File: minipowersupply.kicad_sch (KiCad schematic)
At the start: 43 parts, among them J1 Conn_01x08_Female, J2 Conn_01x08_Female, J3 Conn_01x03_Female, J4 Conn_01x08_Female, J5 Conn_01x03_Female, J6 Conn_01x08_Female, J7 Conn_01x03_Female, J8 Conn_01x02_Female, J9 Conn_01x02_Female, Q1 BC817, U1 LM7805_TO220, U15 LT1084-3.3, U2 LM317L_TO92, U3 LM337L_TO92, U4 CD74HC4067SM

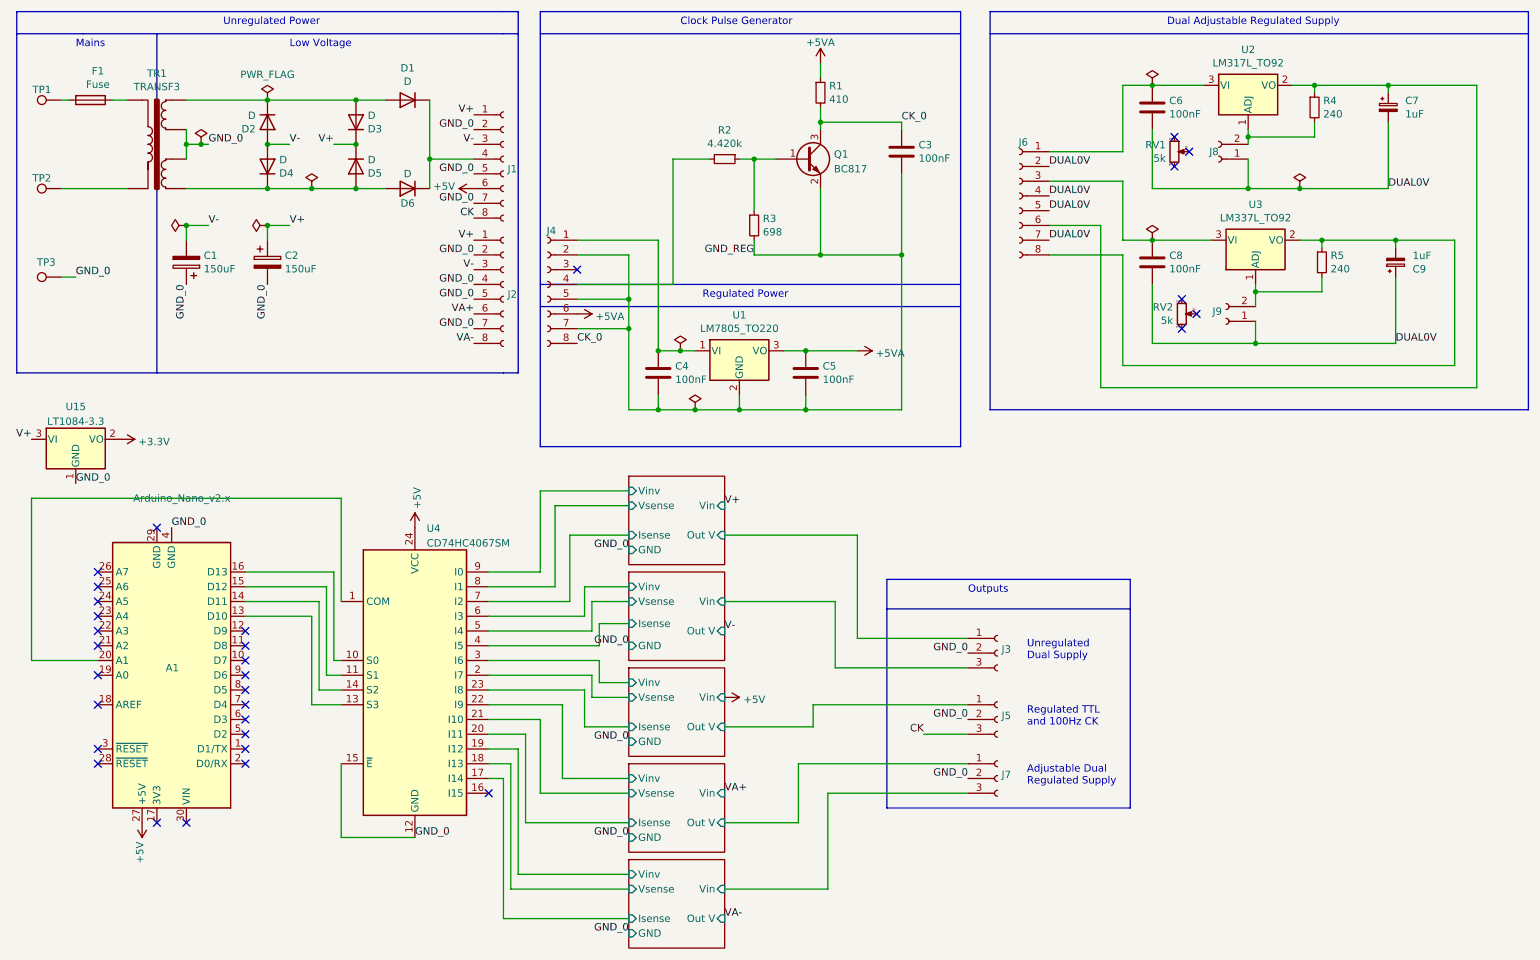
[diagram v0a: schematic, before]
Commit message: finalising diagram
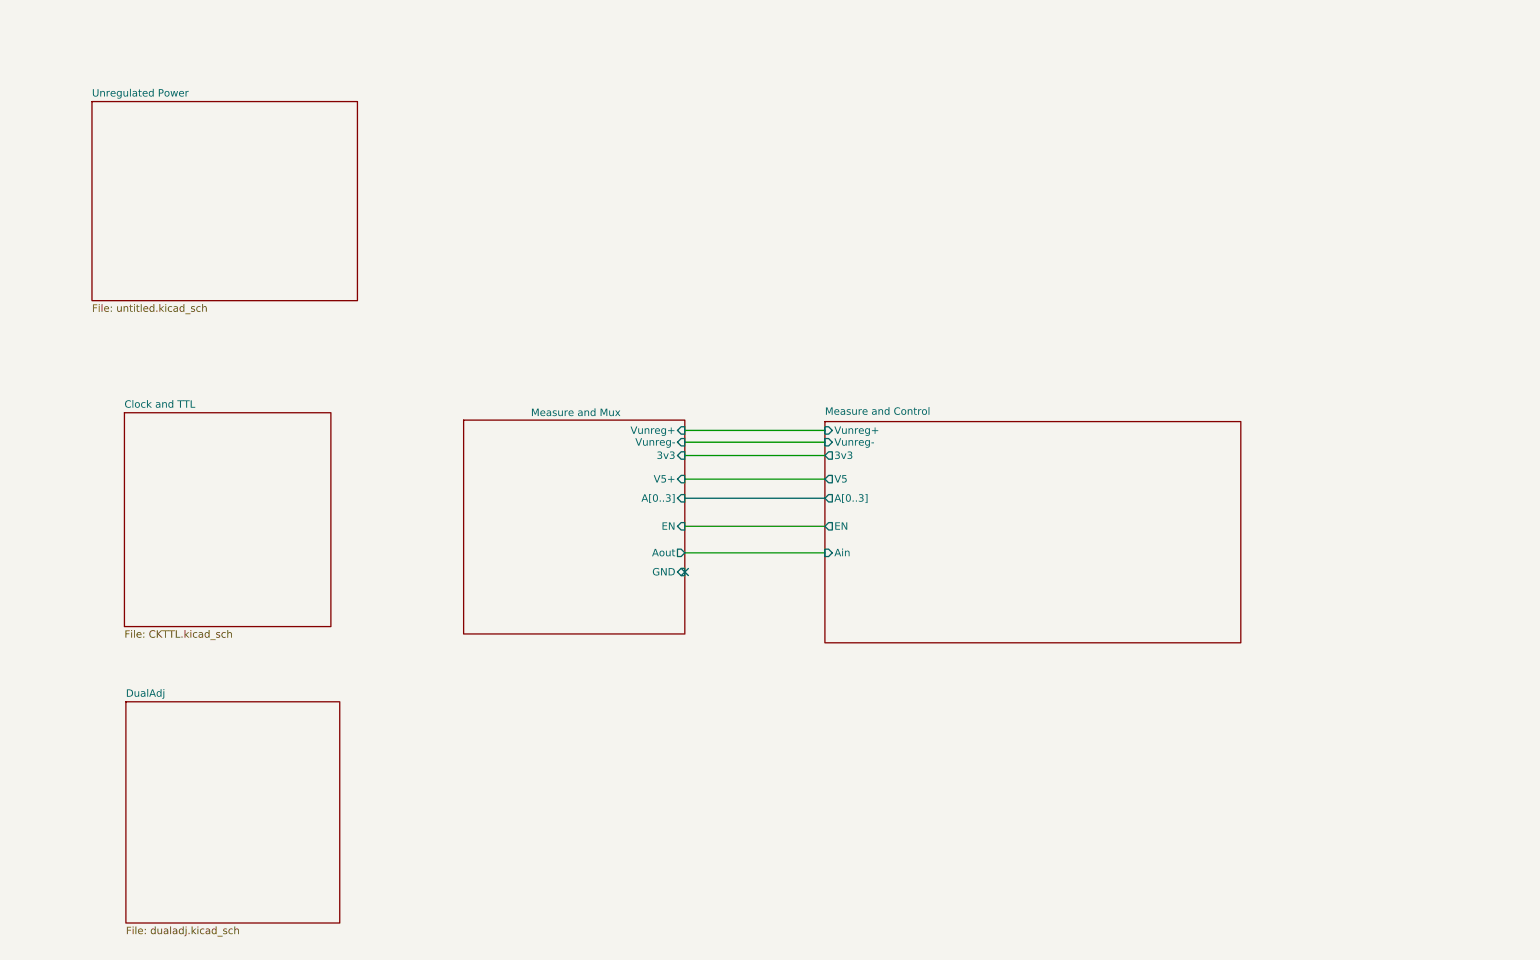
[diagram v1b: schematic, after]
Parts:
- removed A1: Arduino_Nano_v2.x, Module:Arduino_Nano, symbol MCU_Module:Arduino_Nano_v2.x
- removed C1, C2: 150uF, Capacitor_THT:CP_Radial_D8.0mm_P3.50mm, symbol minipowersupply-rescue:CP-Device
- removed C3, C4, C5, C6, C8: 100nF, Capacitor_THT:C_Disc_D8.0mm_W5.0mm_P5.00mm, symbol Device:C
- removed C7, C9: 1uF, Capacitor_THT:C_Disc_D8.0mm_W5.0mm_P5.00mm, symbol Device:C_Polarized_Small
- removed D1, D2, D3, D4, D5, D6: D, Diode_THT:D_T-1_P10.16mm_Horizontal, symbol Device:D
- removed F1: Fuse, Fuse:Fuseholder_Cylinder-5x20mm_Bulgin_FX0457_Horizontal_Closed, symbol Device:Fuse
- removed J1, J2, J4, J6: Conn_01x08_Female, Connector_PinHeader_2.54mm:PinHeader_1x08_P2.54mm_Vertical, symbol Connector:Conn_01x08_Female
- removed J3, J5, J7: Conn_01x03_Female, Connector_PinHeader_2.54mm:PinHeader_1x03_P2.54mm_Vertical, symbol Connector:Conn_01x03_Female
- removed J8, J9: Conn_01x02_Female, Connector_PinHeader_2.54mm:PinHeader_1x02_P2.54mm_Vertical, symbol Connector:Conn_01x02_Female
- removed Q1: BC817, Package_TO_SOT_SMD:SOT-23, symbol Transistor_BJT:BC817
- removed R1: 410, Resistor_THT:R_Axial_DIN0207_L6.3mm_D2.5mm_P5.08mm_Vertical, symbol Device:R_Small
- removed R2: 4.420k, Resistor_THT:R_Axial_DIN0207_L6.3mm_D2.5mm_P5.08mm_Vertical, symbol Device:R_Small
- removed R3: 698, Resistor_THT:R_Axial_DIN0207_L6.3mm_D2.5mm_P5.08mm_Vertical, symbol Device:R_Small
- removed R4, R5: 240, Resistor_THT:R_Axial_DIN0207_L6.3mm_D2.5mm_P5.08mm_Vertical, symbol Device:R_Small
- removed RV1, RV2: 5k, symbol minipowersupply-rescue:R_POT_Small-Device
- removed TP1, TP2, TP3: TestPoint, TestPoint:TestPoint_THTPad_4.0x4.0mm_Drill2.0mm, symbol Connector:TestPoint
- removed TR1: TRANSF3, minipowersupply:vtxtfr, symbol Transformer:TRANSF3
- removed U1: LM7805_TO220, Package_TO_SOT_SMD:SOT-223-3_TabPin2, symbol Regulator_Linear:LM7805_TO220
- removed U15: LT1084-3.3, symbol Regulator_Linear:LT1084-3.3
- removed U2: LM317L_TO92, Package_TO_SOT_THT:TO-92_Inline, symbol Regulator_Linear:LM317L_TO92
- removed U3: LM337L_TO92, Package_TO_SOT_THT:TO-92_Inline, symbol Regulator_Linear:LM337L_TO92
- removed U4: CD74HC4067SM, Package_SO:SSOP-24_5.3x8.2mm_P0.65mm, symbol 74xx:CD74HC4067SM
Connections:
- no-connect marks 31 -> 1
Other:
- removed sheet Curent and Volt4
- removed sheet Curent and Volt5
- removed sheet Curent and Volt6
- removed sheet Curent and Volt7
- removed sheet Curent and Volt8
- added sheet  Measure and Mux (arduino.kicad_sch)
- added sheet Clock and TTL (CKTTL.kicad_sch)
- added sheet DualAdj (dualadj.kicad_sch)
- added sheet Measure and Control (MAC.kicad_sch)
- added sheet Unregulated Power (untitled.kicad_sch)
- note removed: "Adjustable Dual Regulated Supply"
- note removed: "Clock Pulse Generator"
- note removed: "Dual Adjustable Regulated Supply"
- note removed: "Low Voltage"
- note removed: "Mains"
- note removed: "Outputs"
- note removed: "Regulated Power"
- note removed: "Regulated TTL and 100Hz CK"
- note removed: "Unregulated Dual Supply"
- note removed: "Unregulated Power"
